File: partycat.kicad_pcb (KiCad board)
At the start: 2 copper layers, 68 x 30 mm, 20 parts, among them P4 CONN_01X06, P6 CONN_01X10, Q2 Q_NMOS_GDS, U1 AP1117, U2 ESP-12, U3 SN54AHCT125

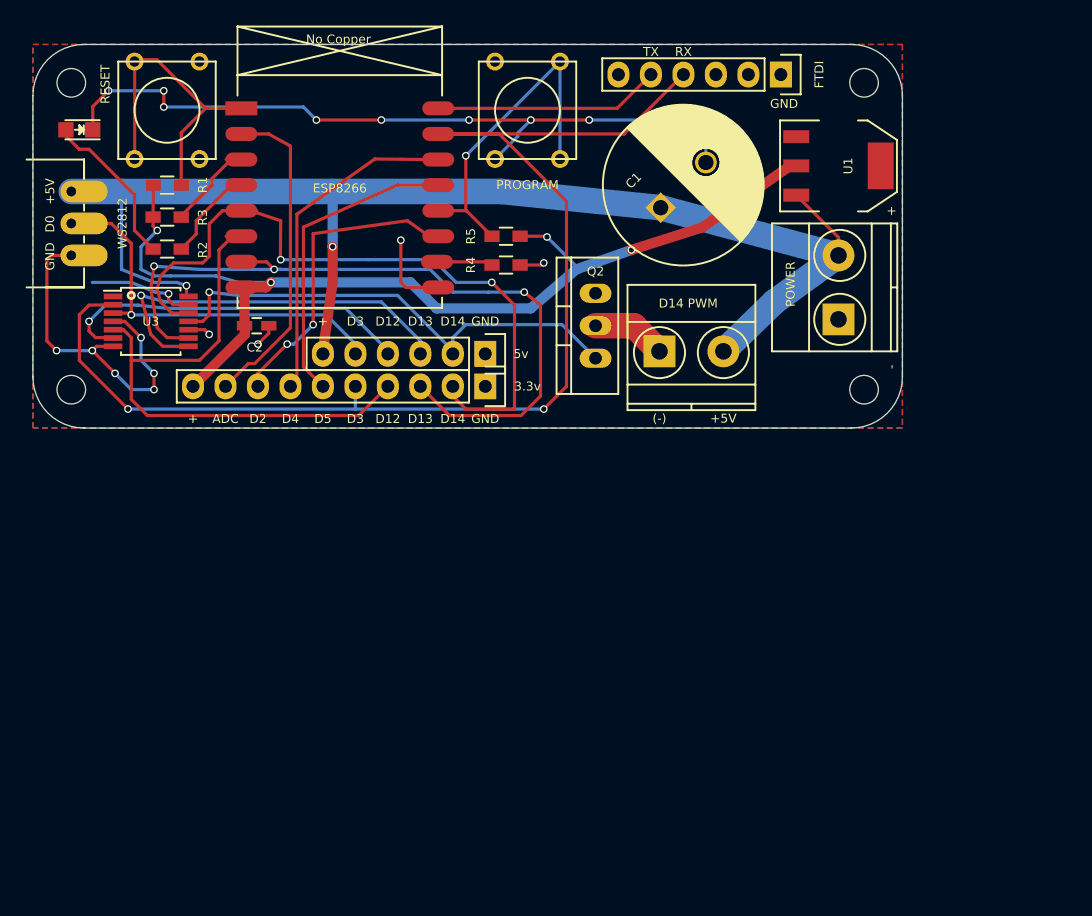
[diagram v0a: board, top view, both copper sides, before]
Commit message: v4
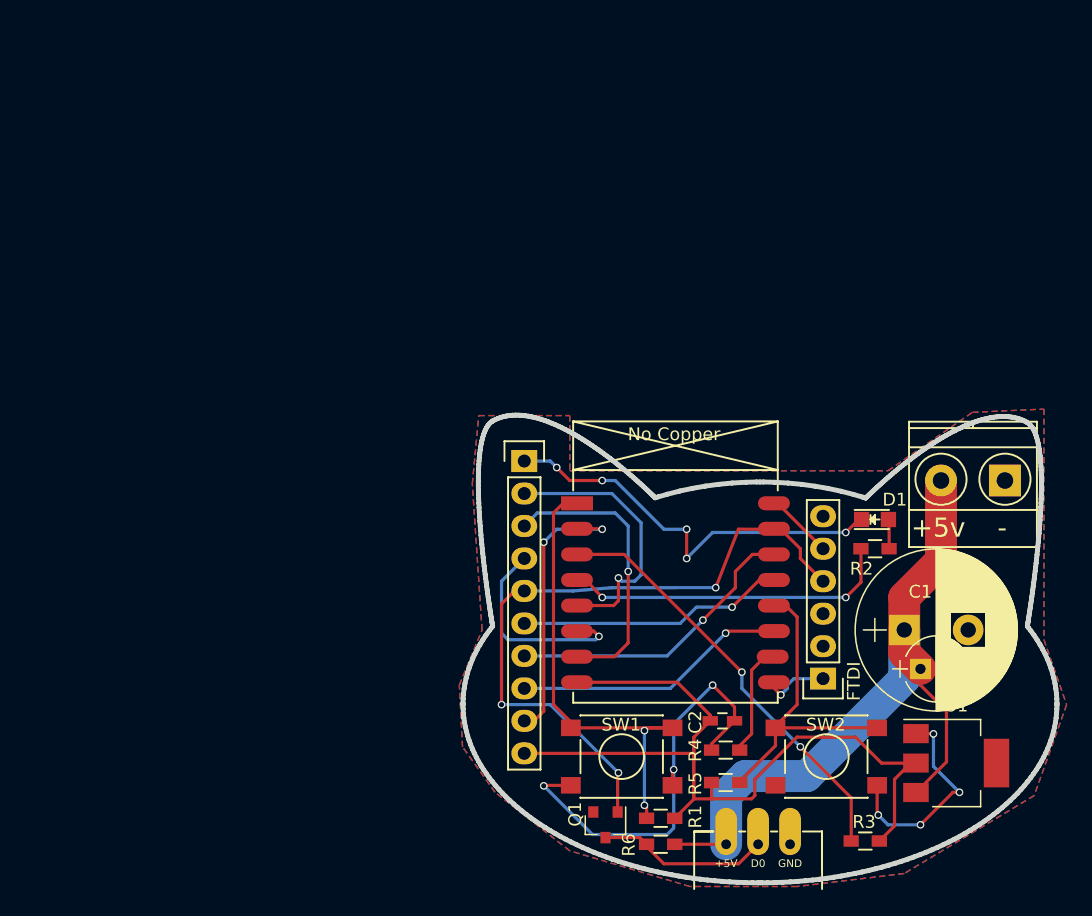
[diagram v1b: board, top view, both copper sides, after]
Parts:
- removed D14 PWM: CONN_01X02, Terminal_Blocks:TerminalBlock_Pheonix_MKDS1.5-2pol
- removed P4: CONN_01X06, Pin_Headers:Pin_Header_Straight_1x06
- removed POWER: CONN_01X02, Terminal_Blocks:TerminalBlock_Pheonix_MKDS1.5-2pol
- removed PROGRAM, RESET: SW_PUSH, Buttons_Switches_ThroughHole:SW_PUSH_SMALL
- removed Q2: Q_NMOS_GDS, TO_SOT_Packages_THT:TO-220_Neutral123_Vertical
- removed U3: SN54AHCT125, Housings_SSOP:TSSOP-14_4.4x5mm_Pitch0.65mm
- removed WS2812: CONN_01X03, WS2812:WS2812_Strip
- added C3: CP, Capacitors_THT:CP_Radial_D5.0mm_P2.50mm, F.Cu at (137.4, 84.8)
- added P1: CONN_01X02, Terminal_Blocks:TerminalBlock_Pheonix_MKDS1.5-2pol, F.Cu at (144.0, 70.1)
- added P2: CONN_01X03, WS2812:WS2812_Strip, F.Cu at (124.7, 98.6)
- added Q1: BSS138, TO_SOT_Packages_SMD:SOT-23, F.Cu at (112.8, 97.0)
- added R6: 4.7k, Resistors_SMD:R_0603_HandSoldering, F.Cu at (117.1, 98.6)
- added SW1: SW_PUSH, Buttons_Switches_SMD:SW_SPST_PTS645, F.Cu at (114.0, 91.7)
- added SW2: SW_PUSH, Buttons_Switches_SMD:SW_SPST_PTS645, F.Cu at (130.0, 91.7)
- C1: footprint Capacitors_ThroughHole:C_Radial_D12.5_L25_P5 -> Capacitors_THT:CP_Radial_D12.5mm_P5.00mm
- moved R3 73.2 mm to (133.1, 98.3), turned to 0 degrees
- moved D1 69.3 mm to (133.9, 73.2), turned to 0 degrees
- moved R1 62.8 mm to (117.1, 96.5), turned to 0 degrees
- moved R2 60.1 mm to (133.9, 75.4), turned to 180 degrees
- moved C2 47.8 mm to (121.9, 88.9)
- moved U1 47.6 mm to (140.2, 92.2), turned to 0 degrees
- moved FTDI 47.4 mm to (129.8, 85.6), turned to 180 degrees
- moved R5 46.0 mm to (122.2, 93.7), turned to 0 degrees
- moved R4 41.6 mm to (122.2, 91.2), turned to 0 degrees
- moved U2 40.5 mm to (111.3, 71.9)
- moved C1 38.1 mm to (136.1, 81.8), turned to 0 degrees
- moved P6 6.59 mm to (106.4, 68.6), turned to 0 degrees
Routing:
- net +5V: track 103.2 -> 57.3 mm, vias 2 -> 0
- net Net-(P3-Pad4): track 98.9 -> 53.2 mm, vias 2 -> 3
- net Net-(P6-Pad3): track 60.8 -> 21.9 mm, vias 3 -> 1
- net Net-(P4-Pad2): track 38.2 -> 0.00 mm, vias 1 -> 0
- net Net-(P6-Pad2): track 56.4 -> 20.7 mm, vias 2 -> 1
- net Net-(P6-Pad4): track 49.7 -> 15.7 mm, vias 0 -> 1
- net Net-(P4-Pad3): track 30.4 -> 0.00 mm, vias 1 -> 0
- net Net-(P4-Pad4): track 28.1 -> 0.00 mm, vias 1 -> 0
- net Net-(R3-Pad1): track 9.52 -> 32.8 mm, vias 0 -> 2
- net GND: track 108.9 -> 89.0 mm, vias 19 -> 13
- net Net-(P2-Pad2): track 31.4 -> 13.5 mm, vias 1 -> 0
- net Net-(R2-Pad2): track 9.98 -> 25.2 mm, vias 0 -> 2
- net Net-(P3-Pad5): track 18.4 -> 6.01 mm
- net +3V3: track 79.8 -> 68.0 mm, vias 4 -> 0
- net Net-(D1-Pad2): track 12.7 -> 2.31 mm
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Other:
- board size 68 x 30 mm -> 46.5 x 36.6 mm
- net class MiniPower removed
- net class Power removed
- rule pad_to_mask_clearance: 0 -> 0.2
- board text added: "+3.3v"
- board text added: "+5v"
- board text added: "12"
- board text added: "13"
- board text added: "14"
- board text added: "2"
- board text added: "3"
- board text added: "4"
- board text added: "5"
- board text added: "partycat"
- board text added: "rev 4 • December 2017 Luke Cyca"
- board text removed: "(-)"
- board text removed: "+"
- board text removed: "+5V"
- board text removed: "3.3v"
- board text removed: "5v"
- board text removed: "D12"
- board text removed: "D13"
- board text removed: "D14"
- board text removed: "D2"
- board text removed: "D3"
- board text removed: "D4"
- board text removed: "D5"
- board text removed: "ESP8266"
- board text removed: "LUKE CYCA • 2016-11-26 • rev 3"
- board text removed: "RX"
- board text removed: "TX"
- board text removed: "light controller"
- board text removed: "party cat"
